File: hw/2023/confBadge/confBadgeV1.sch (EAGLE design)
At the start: 84 parts, among them J1 10118192-0002LF, Q1 8/16/20MHz, U1 ATMEGA328, U10 WS2812-2020, U11 WS2812-2020, U12 WS2812-2020, U13 WS2812-2020, U14 WS2812-2020, U15 WS2812-2020, U16 WS2812-2020, U17 WS2812-2020, U18 WS2812-2020, U19 WS2812-2020, U2 AP2112-3.3, U20 WS2812-2020, U21 WS2812-2020, U22 WS2812-2020, U3 WS2812-2020, U4 WS2812-2020, U5 PCM12SMTRPCM12SMTR_CNK, U6 24792479PCB_37P49X52P63_KEY, U7 CH340C, U8 SMF05CT1G, U9 WS2812-2020

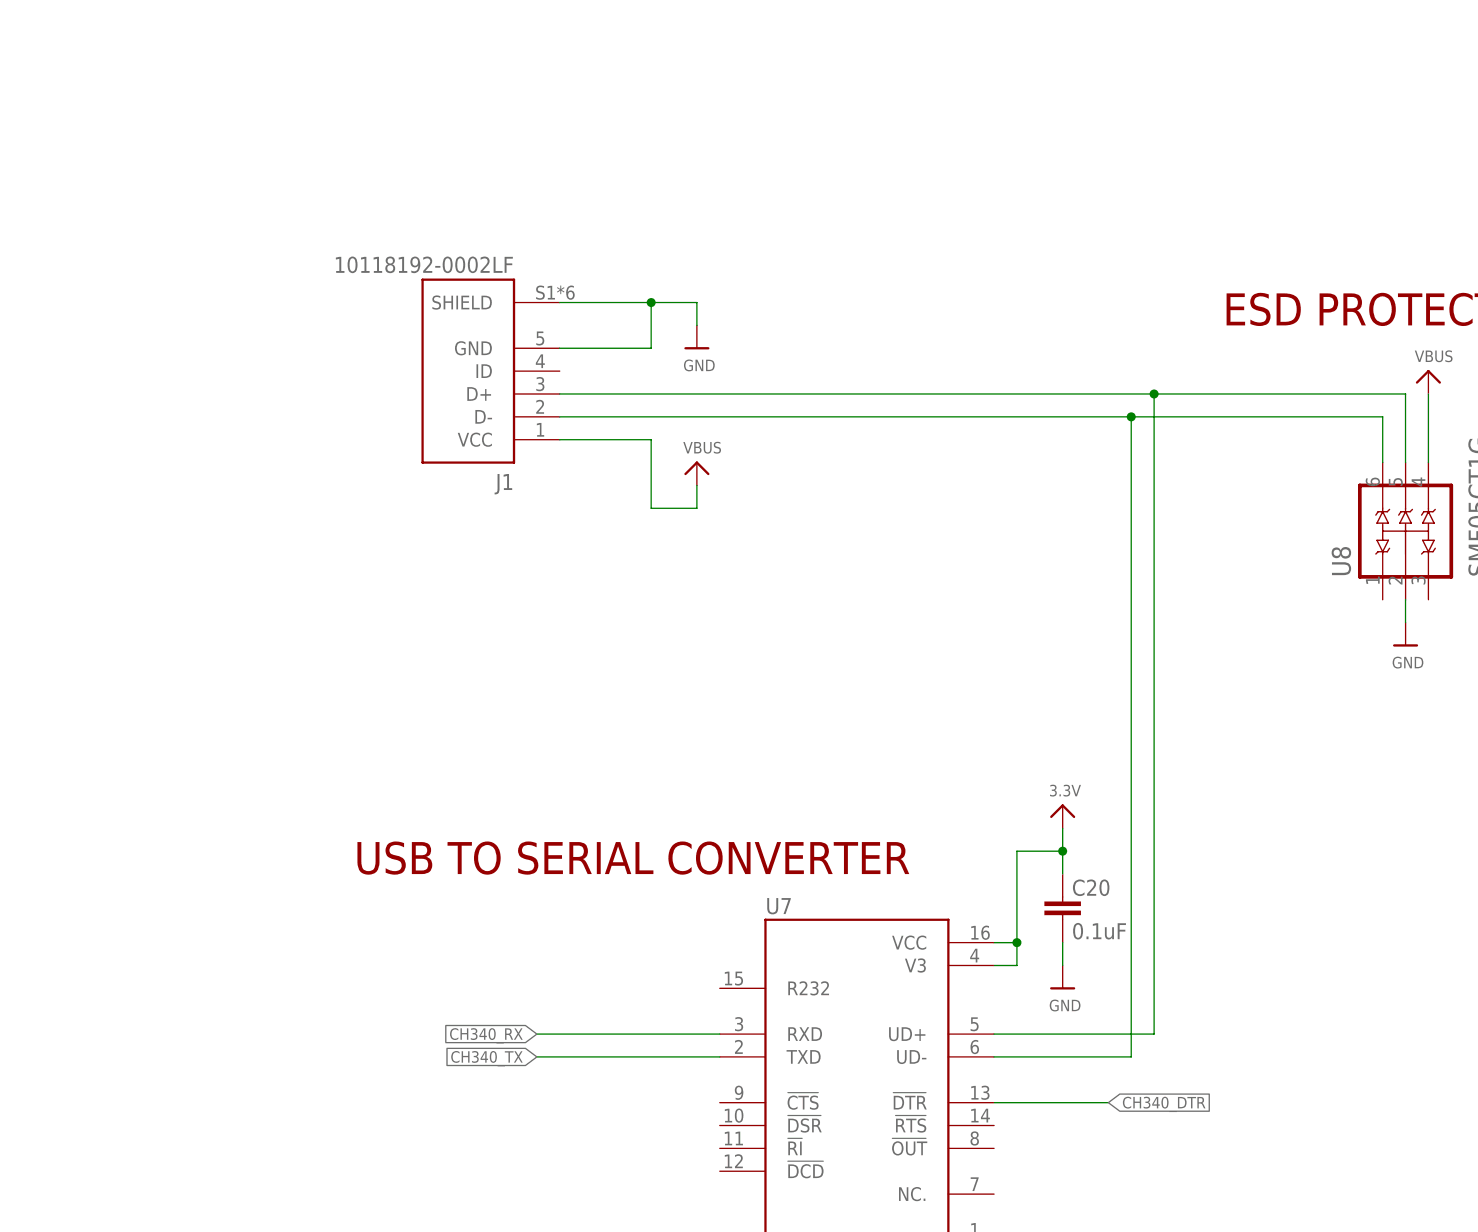
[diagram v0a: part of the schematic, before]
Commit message: Switch to USB-C for both badge
ctf-badge
- switched to USB-C
- switched to smaller neopixel
- switched to 3xAAA
- removed lipo charging circuit
conf-badge
- switched to USB-C
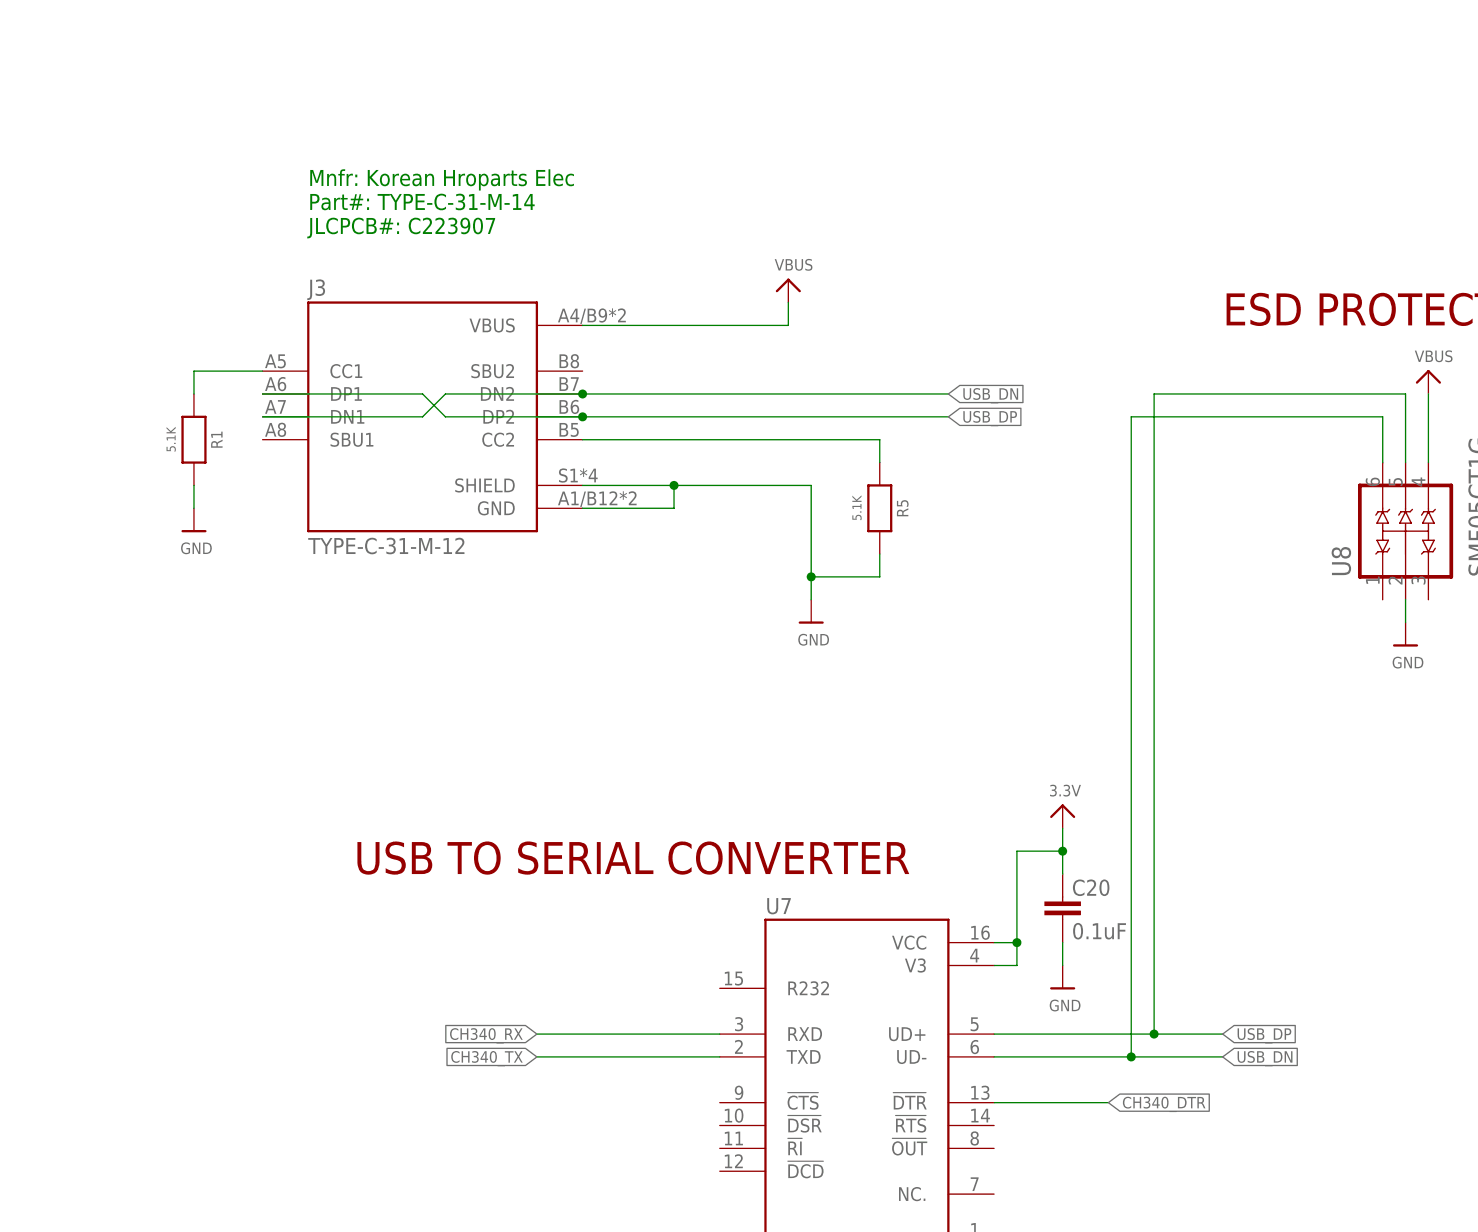
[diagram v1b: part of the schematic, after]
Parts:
- removed J1: 10118192-0002LF, 10118192-0002LF:10118192-0002LF
- added J3: TYPE-C-31-M-12, TYPE-C-31-M-12:TYPE-C-31-M-12
- added R1, R5: 5.1K, microbuilder:RESISTOR_0603_NOOUT
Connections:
- removed net N$28: J1.D+, U7.UD+, U8.C4
- removed net N$29: J1.D-, U7.UD-, U8.C5
- new net N$27: J3.CC2, R5.1
- new net N$30: J3.CC1, R1.1
- new net USB_DN: J3.DN1, J3.DN2, U7.UD-, U8.C5
- new net USB_DP: J3.DP1, J3.DP2, U7.UD+, U8.C4
- net GND: now also J3.GND, J3.SHIELD, R1.2, R5.2; no longer J1.GND, J1.SHIELD
- net VBUS: now also J3.VBUS; no longer J1.VCC
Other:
- note added: "Mnfr: Korean Hroparts Elec Part#: TYPE-C-31-M-14 JLCPCB#: C223907"
